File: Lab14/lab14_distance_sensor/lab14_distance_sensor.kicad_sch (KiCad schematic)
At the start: 0 parts

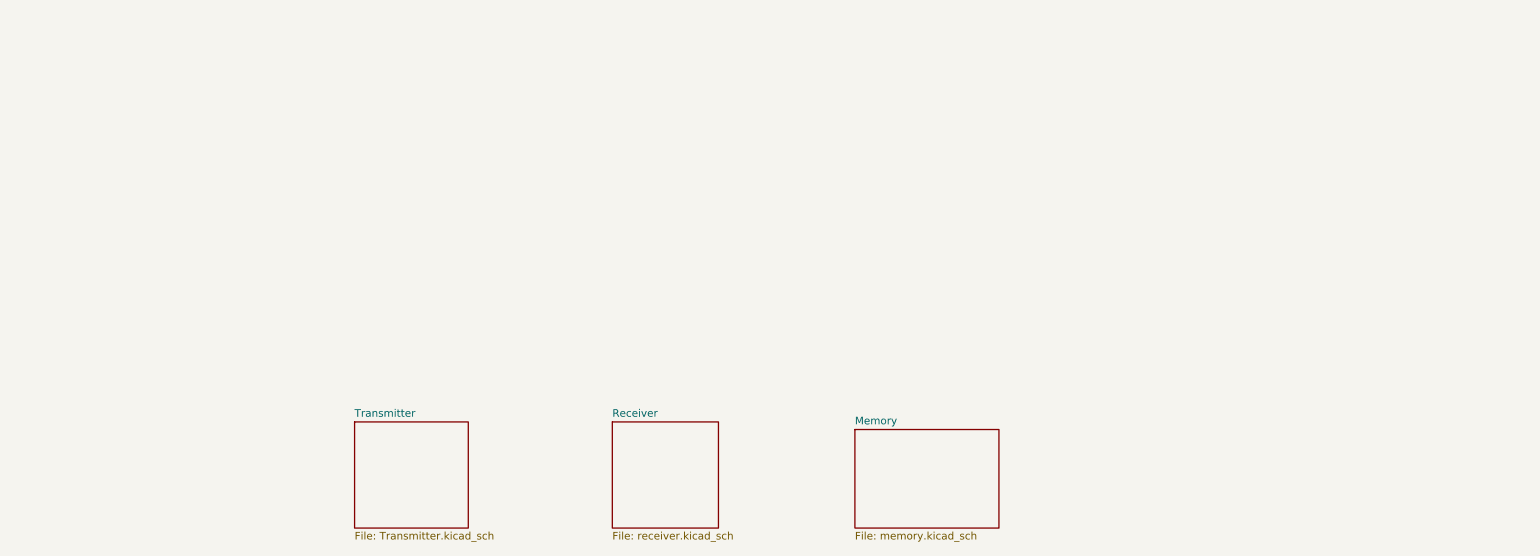
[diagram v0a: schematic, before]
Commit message: work on lab 14
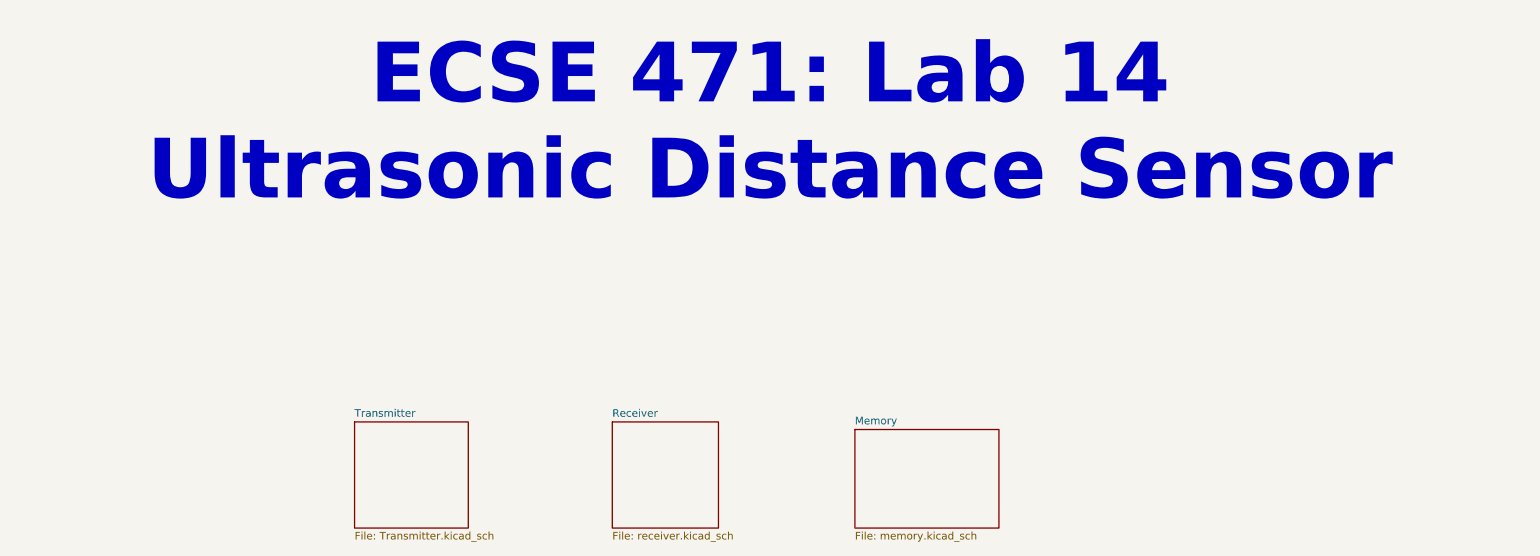
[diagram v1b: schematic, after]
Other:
- note added: "ECSE 471: Lab 14 Ultrasonic Distance Sensor"
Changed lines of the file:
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@@
 	(generator_version "8.0")
 	(paper "A4")
+	(text "ECSE 471: Lab 14 \nUltrasonic Distance Sensor "
+		(exclude_from_sim no)
+		(at 153.416 43.942 0)
+		(effects
+			(font
+				(size 10 10)
+				(thickness 2)
+				(bold yes)
+			)
+		)
+	)
 	(sheet
 		(at 127 93.98)
